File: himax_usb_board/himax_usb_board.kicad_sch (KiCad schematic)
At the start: 10 parts

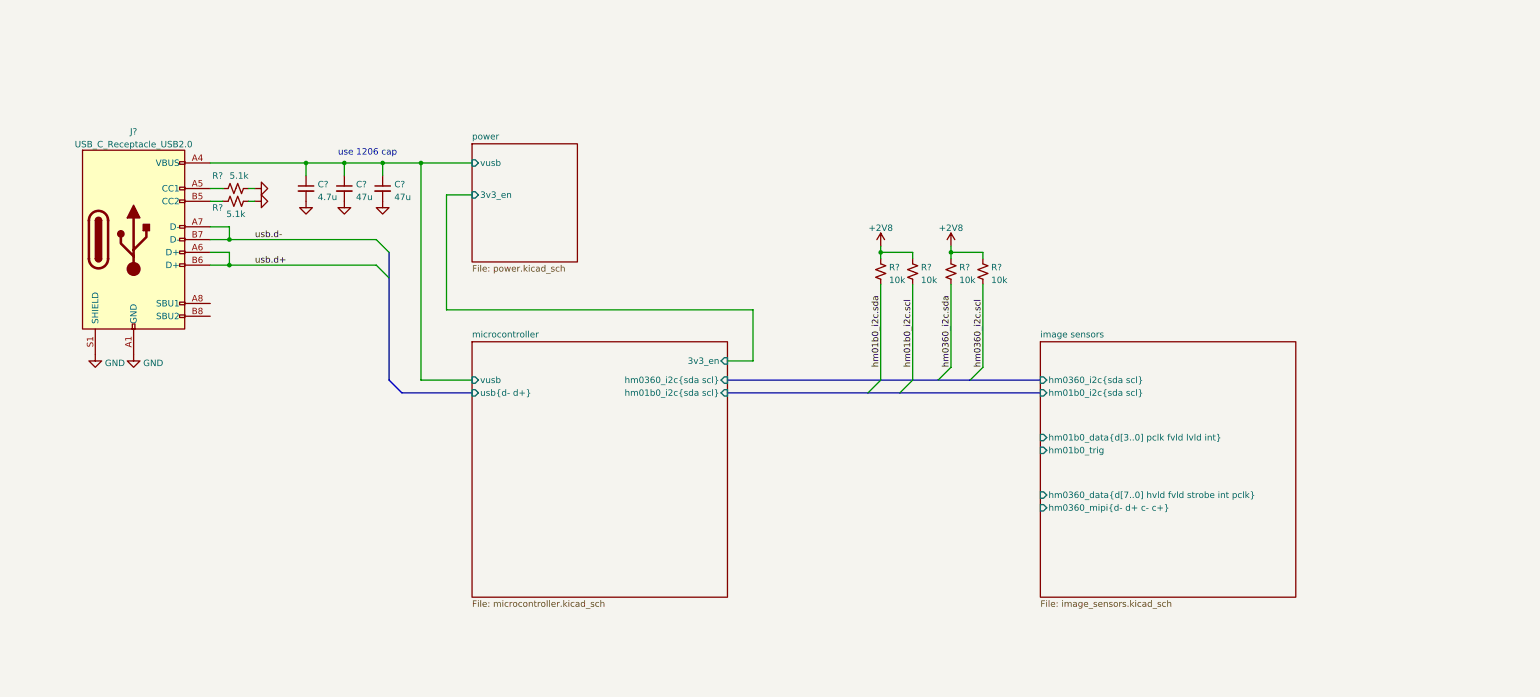
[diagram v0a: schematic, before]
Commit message: schematic wip
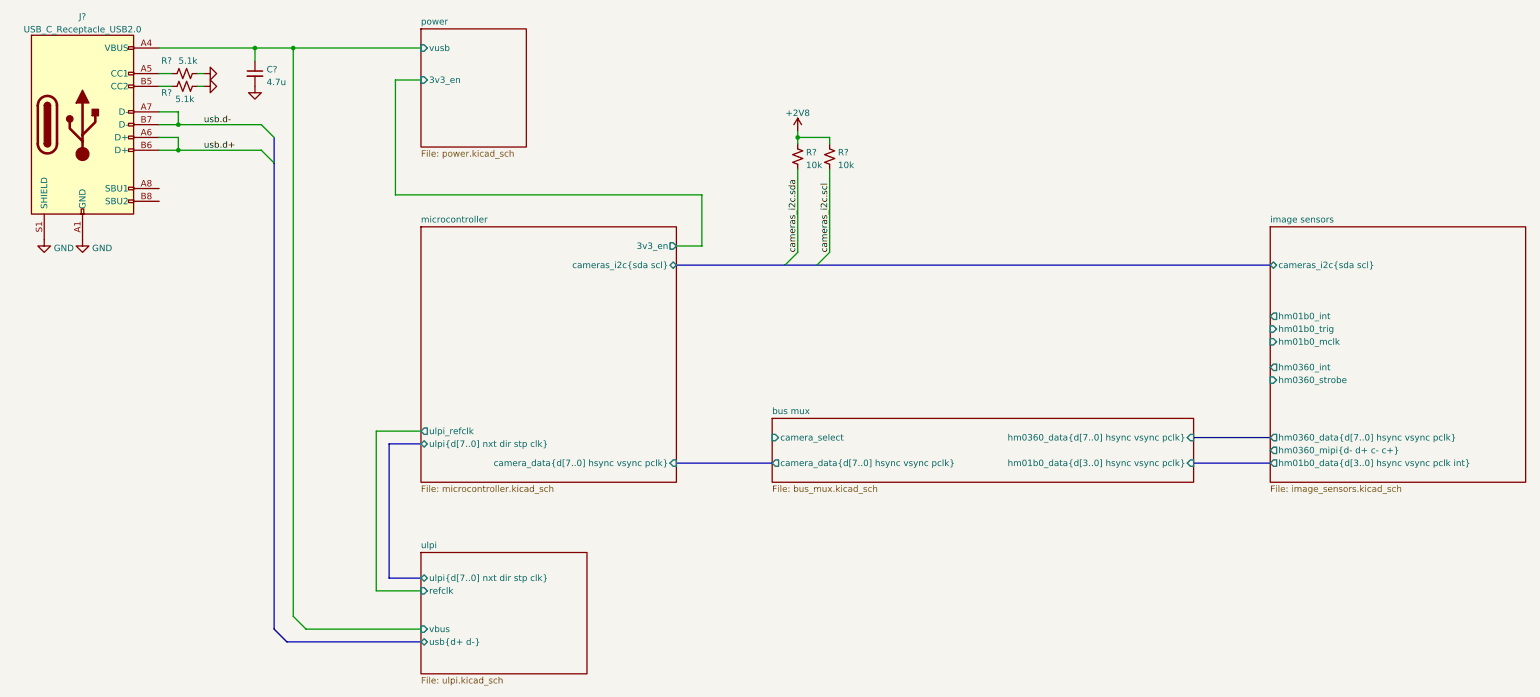
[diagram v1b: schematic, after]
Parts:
- removed C? (x2): 47u, symbol Device:C_Small
- removed R? (x2): 10k, symbol Device:R_Small_US
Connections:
- net hm0360_i2c.scl renamed cameras_i2c.scl
- net hm0360_i2c.sda renamed cameras_i2c.sda
- net microcontroller/vusb renamed power/vusb
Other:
- added sheet bus mux (bus_mux.kicad_sch)
- added sheet ulpi (ulpi.kicad_sch)
- sheet image sensors ports: added cameras_i2c{sda scl}, hm01b0_data{d[3..0] hsync vsync pclk int}, hm01b0_int, hm01b0_mclk, hm0360_data{d[7..0] hsync vsync pclk}, hm0360_int, hm0360_strobe; removed hm01b0_data{d[3..0] pclk fvld lvld int}, hm01b0_i2c{sda scl}, hm0360_data{d[7..0] hvld fvld strobe int pclk}, hm0360_i2c{sda scl}
- sheet microcontroller ports: added camera_data{d[7..0] hsync vsync pclk}, cameras_i2c{sda scl}, ulpi_refclk, ulpi{d[7..0] nxt dir stp clk}; removed hm01b0_i2c{sda scl}, hm0360_i2c{sda scl}, usb{d- d+}, vusb
- note removed: "use 1206 cap"
- moved on the sheet: C?, J?, R?
